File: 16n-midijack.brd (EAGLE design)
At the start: 248.9 x 101.6 mm, 28 parts

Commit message: Everything on the board.
Now needs routing. Oh boy.
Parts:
- added C1, C2, C3, C4, C5, C6, C7, C8: 100n, rcl:C0805
- added J1, J10, J11, J12, J13, J14, J15, J16, J2, J3, J4, J5, J6, J7, J8, J9: THONKICONNNEW, MusicThingModular:WQP-PJ301M-12_JACK
- added R10, R14, R15, R19, R20, R24, R25, R29, R30, R34, R35, R39, R40, R44, R5, R9: 5.6K, rcl:R0805
- added R11, R13, R16, R18, R21, R23, R26, R28, R31, R33, R36, R38, R41, R43, R6, R8: 10K, rcl:R0805
- added R12, R17, R22, R27, R32, R37, R42, R45, R46, R47, R48, R49, R50, R51, R52, R7: 100, rcl:R0805
- added U1, U2, U3, U4, U5, U6, U7, U8: MCP6004_SMD, MusicThingModular:SO14
- D1, D2, D3, D4: device SparkFun-DiscreteSemi:DIODE-1N4148 -> foxfield:SOD-123
- R1, R2: value (none) -> 220; device SparkFun-Resistors:AXIAL-0.3-KIT -> rcl:R0805
- R3, R4: device SparkFun-Resistors:AXIAL-0.3-KIT -> rcl:R0805
- moved D4 35.3 mm to (46.4, 21.6)
- moved R4 30.3 mm to (43.8, 21.6), turned to 270 degrees
- moved D3 29.0 mm to (48.9, 21.6)
- moved D2 16.7 mm to (54.0, 21.6)
- moved D1 15.5 mm to (51.4, 21.6)
- moved R1 9.69 mm to (228.0, 11.4)
- moved R3 7.65 mm to (56.5, 21.6), turned to 270 degrees
- moved R2 5.12 mm to (224.2, 11.4)
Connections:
- new net CV1: J1.P$1_TIP, R7.2
- new net CV10: J10.P$1_TIP, R48.2
- new net CV11: J11.P$1_TIP, R32.2
- new net CV12: J12.P$1_TIP, R49.2
- new net CV13: J13.P$1_TIP, R37.2
- new net CV14: J14.P$1_TIP, R50.2
- new net CV15: J15.P$1_TIP, R42.2
- new net CV16: J16.P$1_TIP, R51.2
- new net CV2: J2.P$1_TIP, R12.2
- new net CV3: J3.P$1_TIP, R52.2
- new net CV4: J4.P$1_TIP, R45.2
- new net CV5: J5.P$1_TIP, R17.2
- new net CV6: J6.P$1_TIP, R47.2
- new net CV7: J7.P$1_TIP, R22.2
- new net CV8: J8.P$1_TIP, R46.2
- new net CV9: J9.P$1_TIP, R27.2
- new net N$10: R8.2, R9.2, U1.12
- new net N$11: R17.1, U3.8, U3.9
- new net N$12: R15.2, R16.2, U3.10
- new net N$13: R18.2, R19.2, U3.12
- new net N$14: R22.1, U4.8, U4.9
- new net N$15: R20.2, R21.2, U4.10
- new net N$16: R23.2, R24.2, U4.12
- new net N$17: R27.1, U5.8, U5.9
- new net N$18: R25.2, R26.2, U5.10
- new net N$19: R28.2, R29.2, U5.12
- new net N$20: R32.1, U6.8, U6.9
- new net N$21: R30.2, R31.2, U6.10
- new net N$22: R33.2, R34.2, U6.12
- new net N$23: R37.1, U7.8, U7.9
- new net N$24: R35.2, R36.2, U7.10
- new net N$25: R38.2, R39.2, U7.12
- new net N$256: R12.1, U1.13, U1.14
- new net N$257: R45.1, U2.13, U2.14
- new net N$258: R47.1, U3.13, U3.14
- new net N$259: R46.1, U4.13, U4.14
- new net N$26: R42.1, U8.8, U8.9
- new net N$260: R48.1, U5.13, U5.14
- new net N$261: R49.1, U6.13, U6.14
- new net N$262: R50.1, U7.13, U7.14
- new net N$263: R51.1, U8.13, U8.14
- new net N$27: R40.2, R41.2, U8.10
- new net N$28: R43.2, R44.2, U8.12
- new net N$5: R52.1, U2.8, U2.9
- new net N$6: R10.2, R11.2, U2.10
- new net N$7: R13.2, R14.2, U2.12
- new net N$8: R7.1, U1.8, U1.9
- new net N$9: R5.2, R6.2, U1.10
- new net W0: R5.1, U$17.2, U1.5
- new net W1: R9.1, U$16.2, U1.3
- new net W10: R30.1, U$7.2, U6.5
- new net W11: R34.1, U$6.2, U6.3
- new net W12: R35.1, U$5.2, U7.5
- new net W13: R39.1, U$4.2, U7.3
- new net W14: R40.1, U$3.2, U8.5
- new net W15: R44.1, U$2.2, U8.3
- new net W2: R10.1, U$15.2, U2.5
- new net W3: R14.1, U$14.2, U2.3
- new net W4: R15.1, U$13.2, U3.5
- new net W5: R19.1, U$12.2, U3.3
- new net W6: R20.1, U$11.2, U4.5
- new net W7: R24.1, U$10.2, U4.3
- new net W8: R25.1, U$9.2, U5.5
- new net W9: R29.1, U$8.2, U5.3
- net +3V3: now also R3.2, R4.2; no longer R3.P$2, R4.P$2, U$10.1, U$11.1, U$12.1, U$13.1, U$14.1, U$15.1, U$16.1, U$17.1, U$2.1, U$3.1, U$4.1, U$5.1, U$6.1, U$7.1, U$8.1, U$9.1
- net +5V: now also C1.1, C2.1, C3.1, C4.1, C5.1, C6.1, C7.1, C8.1, R1.2, U$10.1, U$11.1, U$12.1, U$13.1, U$14.1, U$15.1, U$16.1, U$17.1, U$2.1, U$3.1, U$4.1, U$5.1, U$6.1, U$7.1, U$8.1, U$9.1, U1.4, U2.4, U3.4, U4.4, U5.4, U6.4, U7.4, U8.4; no longer R1.P$2
- net A0: now also U1.6, U1.7; no longer U$2.2
- net A1: now also U1.1, U1.2; no longer U$3.2
- net A10: now also U6.6, U6.7; no longer U$12.2
- net A11: now also U6.1, U6.2; no longer U$13.2
- net A12: now also U7.6, U7.7; no longer U$14.2
- net A13: now also U7.1, U7.2; no longer U$15.2
- net A14: now also U8.6, U8.7; no longer U$16.2
- net A15: now also U8.1, U8.2; no longer U$17.2
- net A2: now also U2.6, U2.7; no longer U$4.2
- net A3: now also U2.1, U2.2; no longer U$5.2
- net A4: now also U3.6, U3.7; no longer U$6.2
- net A5: now also U3.1, U3.2; no longer U$7.2
- net A6: now also U4.6, U4.7; no longer U$8.2
- net A7: now also U4.1, U4.2; no longer U$9.2
- net A8: now also U5.6, U5.7; no longer U$10.2
- net A9: now also U5.1, U5.2; no longer U$11.2
- net GND: now also C1.2, C2.2, C3.2, C4.2, C5.2, C6.2, C7.2, C8.2, J1.P$3_SLEEVE, J10.P$3_SLEEVE, J11.P$3_SLEEVE, J12.P$3_SLEEVE, J13.P$3_SLEEVE, J14.P$3_SLEEVE, J15.P$3_SLEEVE, J16.P$3_SLEEVE, J2.P$3_SLEEVE, J3.P$3_SLEEVE, J4.P$3_SLEEVE, J5.P$3_SLEEVE, J6.P$3_SLEEVE, J7.P$3_SLEEVE, J8.P$3_SLEEVE, J9.P$3_SLEEVE, R11.1, R13.1, R16.1, R18.1, R21.1, R23.1, R26.1, R28.1, R31.1, R33.1, R36.1, R38.1, R41.1, R43.1, R6.1, R8.1, U1.11, U2.11, U3.11, U4.11, U5.11, U6.11, U7.11, U8.11
- net MIDI_OUT: now also R2.2; no longer R2.P$2
- net N$3: now also R2.1; no longer R2.P$1
- net N$4: now also R1.1; no longer R1.P$1
- net SCL: now also R4.1; no longer R4.P$1
- net SDA: now also R3.1; no longer R3.P$1
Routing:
- net +5V: track 226.7 -> 822.4 mm, vias 0 -> 9
- net +3V3: track 430.6 -> 81.1 mm, vias 1 -> 0
- net A1: track 231.6 -> 1.27 mm
- net A2: track 218.2 -> 1.27 mm
- net A0: track 245.1 -> 32.3 mm, vias 0 -> 1
- net A3: track 204.7 -> 1.27 mm
- net A4: track 190.5 -> 1.27 mm
- net A6: track 174.8 -> 1.27 mm
- net A5: track 174.2 -> 1.27 mm
- net A7: track 161.4 -> 1.27 mm
- net A8: track 147.9 -> 1.27 mm
- net N$8: track 0.00 -> 143.5 mm, vias 0 -> 2
- net W0: track 0.00 -> 138.4 mm
- net A9: track 135.5 -> 1.27 mm
- net W1: track 0.00 -> 125.2 mm
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- added copper zone on layer 1, net GND
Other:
- board size 248.9 x 101.6 mm -> 248.9 x 120.7 mm
- board text removed: "220R"
- board text removed: "4.7K, 1N4148"

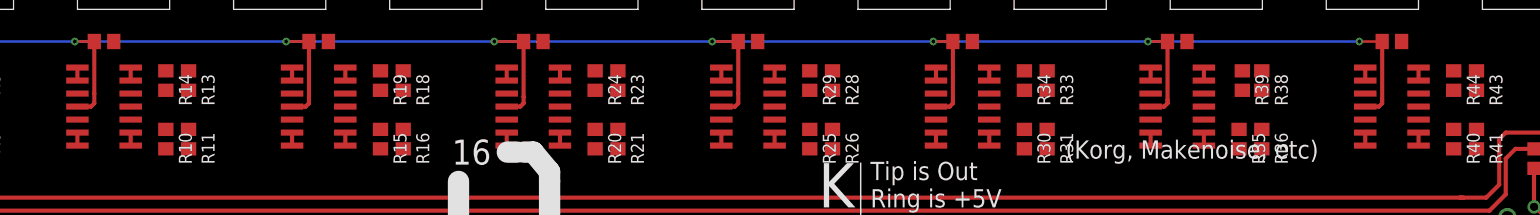
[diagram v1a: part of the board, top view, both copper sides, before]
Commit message: Fixing up some layout.
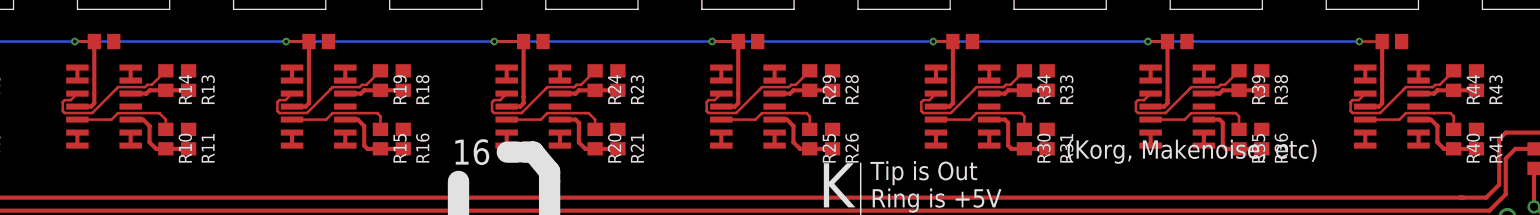
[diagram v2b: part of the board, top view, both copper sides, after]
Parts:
- moved R39 0.32 mm to (195.3, 19.1)
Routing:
- net W11: track 0.00 -> 14.5 mm
- net W7: track 0.00 -> 14.5 mm
- net W15: track 0.00 -> 14.5 mm
- net W5: track 0.00 -> 14.5 mm
- net W3: track 0.00 -> 14.5 mm
- net W13: track 0.00 -> 14.5 mm
- net W9: track 0.00 -> 14.5 mm
- net W8: track 0.00 -> 10.3 mm
- net W14: track 0.00 -> 10.3 mm
- net W12: track 0.00 -> 10.3 mm
- net W4: track 0.00 -> 10.3 mm
- net W10: track 0.00 -> 10.3 mm
- net W6: track 0.00 -> 10.1 mm
- net W2: track 0.00 -> 10.1 mm
- net N$21: track 0.00 -> 8.14 mm
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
